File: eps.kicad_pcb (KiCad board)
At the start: 4 copper layers, 95.9 x 90.2 mm, 185 parts, among them J1 PC104-8BIT, J2 PC104PTH, J3 PC104PTH, J4 PC104PTH, J5 PC104PTH, P1 3pin-DC-power, P2 3pin-DC-power, Q10 CSD17551Q3A, Q11 CSD17551Q3A, Q12 CSD17551Q3A, Q13 CSD25402Q3A, Q14 2N7002ET1G, Q5 DMP3035SFG-7, Q6 DCX124EK-7-F, Q7 2N7002ET1G, Q8 DMP3035SFG-7, Q9 CSD17551Q3A, SW1 LIMIT_SWITCH, SW2 LIMIT_SWITCH, SW3 LIMIT_SWITCH, U1 B3B-XH-A(LF)(SN), U10 CD4555BPWR, U2 TPS563219DDFR-ND, U3 LMS3635AQRNLRQ1, U4 B3B-XH-A(LF)(SN), U5 TPS22967, U6 TPS22967, U7 bq25703arsnt, U9 LM3480

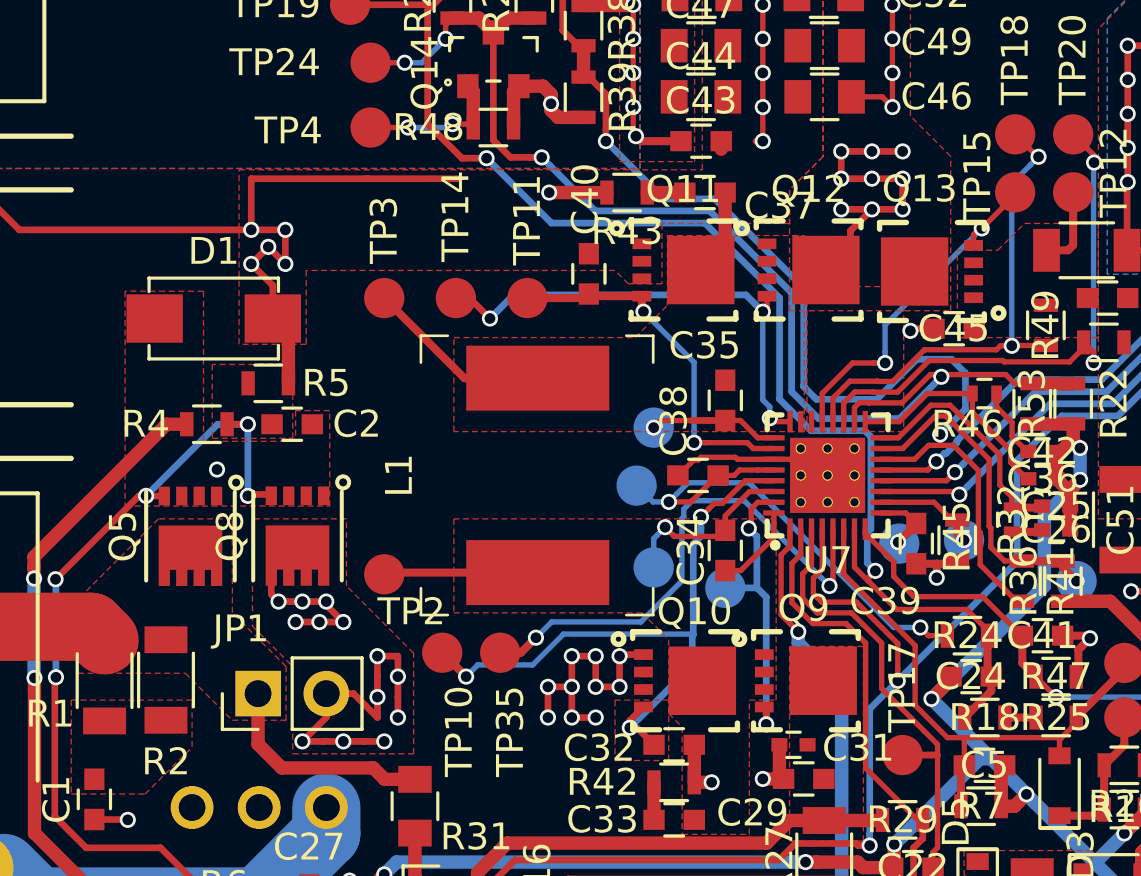
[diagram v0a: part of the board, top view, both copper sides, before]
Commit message: all nets connected
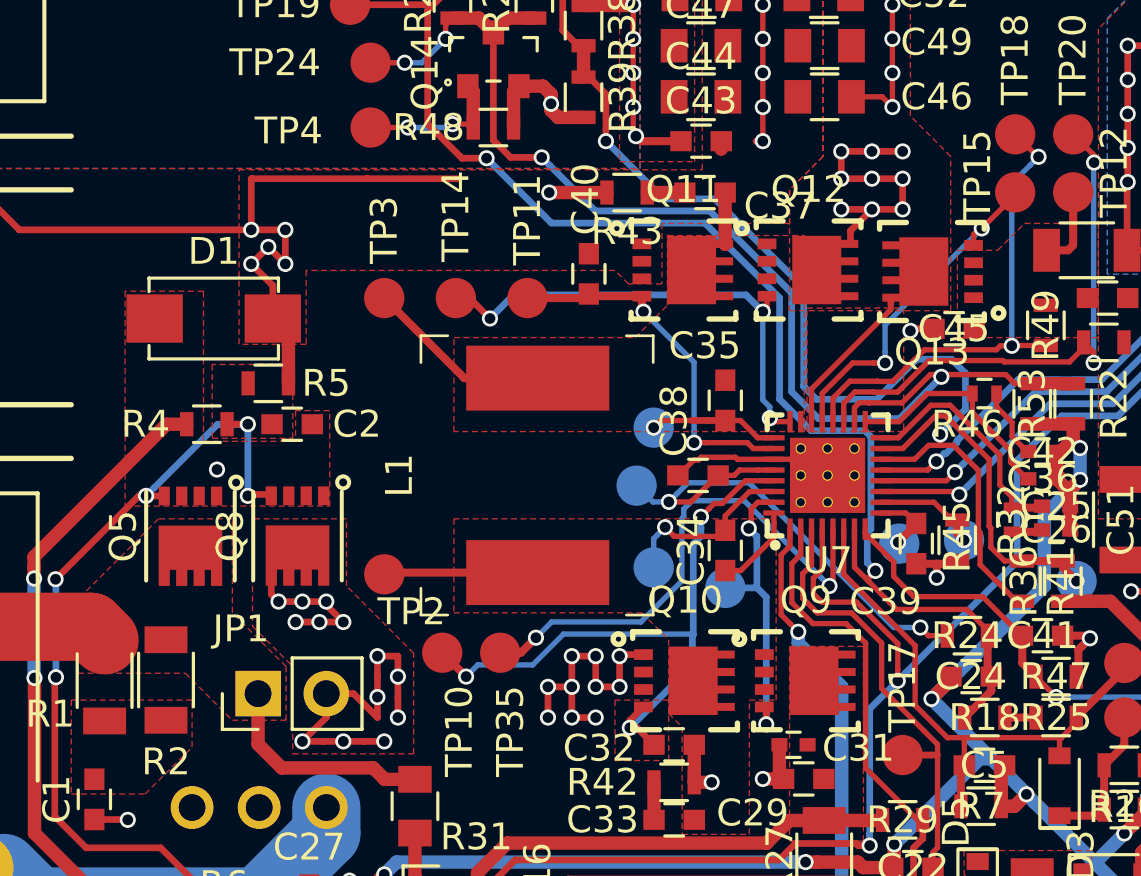
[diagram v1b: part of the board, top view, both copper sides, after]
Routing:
- net /VSYS_UP: track 51.5 -> 57.3 mm
